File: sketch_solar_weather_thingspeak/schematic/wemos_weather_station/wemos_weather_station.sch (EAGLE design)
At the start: 10 parts, among them U1 PHOTORESISTOR-5528-10K

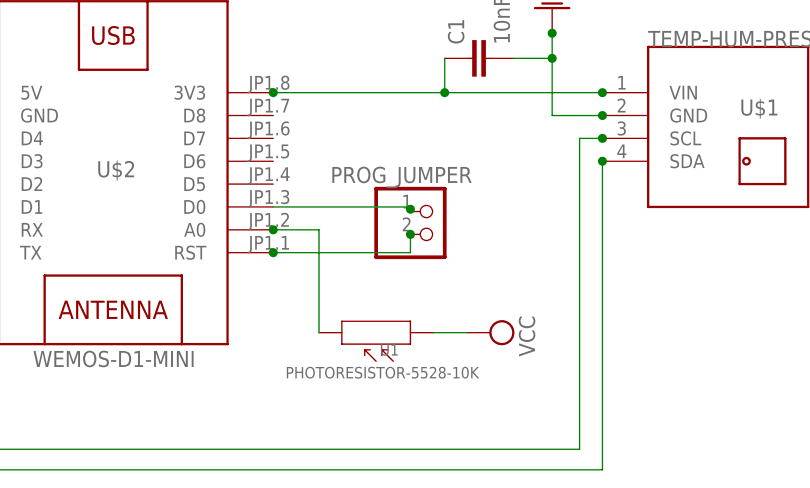
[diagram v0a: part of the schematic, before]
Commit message: schematic updated
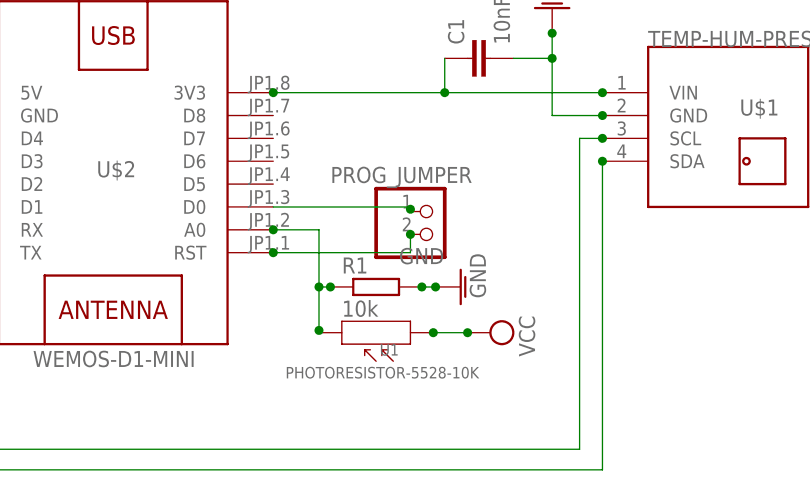
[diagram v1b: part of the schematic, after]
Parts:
- added R1: 10k, resistor:R-EU_0204/7
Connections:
- removed net GNDA: C1.2, C3.1, U$1.GND, U$2.GND, U$3.OUT-
- new net GND: C1.2, C3.1, R1.2, U$1.GND, U$2.GND, U$3.OUT-
- net N$11: now also R1.1
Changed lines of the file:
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@@
 <part name="U1" library="Seeed-Sensor" library_urn="urn:adsk.eagle:library:475" deviceset="PHOTORESISTOR-5528-10K(2P-5.0X4.2MM)" device="" package3d_urn="urn:adsk.eagle:package:32936/1" value="PHOTORESISTOR-5528-10K"/>
 <part name="SUPPLY3" library="supply2" deviceset="VCC" device=""/>
+<part name="R1" library="resistor" library_urn="urn:adsk.eagle:library:348" deviceset="R-EU_" device="0204/7" package3d_urn="urn:adsk.eagle:package:25945/1" value="10k"/>
+<part name="GND3" library="supply1" deviceset="GNDA" device="" value="GND"/>
 </parts>
 <sheets>
@@
 <instance part="SUPPLY3" gate="G$1" x="43.18" y="-10.16" smashed="yes" rot="R270">
 <attribute name="VALUE" x="46.355" y="-8.255" size="1.778" layer="96" rot="R270"/>
+</instance>
+<instance part="R1" gate="G$1" x="30.48" y="-5.08" smashed="yes">
+<attribute name="NAME" x="26.67" y="-3.5814" size="1.778" layer="95"/>
+<attribute name="VALUE" x="26.67" y="-8.382" size="1.778" layer="96"/>
+</instance>
+<instance part="GND3" gate="1" x="39.878" y="-5.08" smashed="yes" rot="R90">
+<attribute name="VALUE" x="42.672" y="-6.35" size="1.778" layer="96" rot="R90"/>
 </instance>
 </instances>
@@
 </segment>
 </net>
-<net name="GNDA" class="0">
+<net name="GND" class="0">
 <segment>
 <pinref part="U$3" gate="G$1" pin="OUT-"/>
@@
 <junction x="-41.402" y="3.302"/>
 </segment>
+<segment>
+<pinref part="GND3" gate="1" pin="GNDA"/>
+<pinref part="R1" gate="G$1" pin="2"/>
+<wire x1="37.338" y1="-5.08" x2="37.084" y2="-5.08" width="0.1524" layer="91"/>
+<junction x="37.084" y="-5.08"/>
+<wire x1="37.084" y1="-5.08" x2="35.56" y2="-5.08" width="0.1524" layer="91"/>
+<junction x="35.56" y="-5.08"/>
+<label x="33.02" y="-2.54" size="1.778" layer="95"/>
+</segment>
 </net>
 <net name="VCC" class="0">
@@
 <pinref part="U1" gate="G$1" pin="P$1"/>
 <wire x1="40.64" y1="-10.16" x2="36.83" y2="-10.16" width="0.1524" layer="91"/>
+<junction x="40.64" y="-10.16"/>
+<junction x="36.83" y="-10.16"/>
 </segment>
 </net>
@@
 <pinref part="U1" gate="G$1" pin="P$2"/>
 <pinref part="U$2" gate="G$1" pin="A0"/>
-<wire x1="24.13" y1="-10.16" x2="24.13" y2="1.27" width="0.1524" layer="91"/>
+<wire x1="24.13" y1="-10.16" x2="24.13" y2="-9.906" width="0.1524" layer="91"/>
+<wire x1="24.13" y1="-9.906" x2="24.13" y2="-5.08" width="0.1524" layer="91"/>
+<wire x1="24.13" y1="-5.08" x2="24.13" y2="1.27" width="0.1524" layer="91"/>
 <wire x1="24.13" y1="1.27" x2="19.05" y2="1.27" width="0.1524" layer="91"/>
 <junction x="19.05" y="1.27"/>
-</segment>
-</net>
+<pinref part="R1" gate="G$1" pin="1"/>
+<wire x1="25.4" y1="-5.08" x2="24.13" y2="-5.08" width="0.1524" layer="91"/>
+<junction x="24.13" y="-5.08"/>
+<junction x="25.4" y="-5.08"/>
+<junction x="24.13" y="-9.906"/>
+</segment>
+</net>
